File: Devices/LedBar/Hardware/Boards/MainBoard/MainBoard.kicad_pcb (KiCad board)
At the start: 2 copper layers, 99 x 24 mm, 115 parts, among them J201 12VDC/5A, J301 RS485, J401 AVR-ISP-6, J501 Left, J502 Center, J503 Right, J601 0-10V(1), Q501 Si2302DS, Q502 Si2302DS, Q503 Si2302DS, Q504 Si2302DS, Q505 Si2302DS, Q506 Si2302DS, Q507 Si2302DS, Q508 Si2302DS, Q509 Si2302DS, Q510 Si2302DS, Q511 Si2302DS, Q512 Si2302DS, Q513 Si2302DS, Q514 Si2302DS, Q515 Si2302DS, Q516 Si2302DS, SW401 reset, U201 INA219AxD, U202 AMS1117-5.0, U301 ISO3082DW, U302 B0505S-1W-SIP4, U401 ATmega48PV-10AU-arduino, U501 PCA9685PW, U701 LM393, Y401 14.7456Mhz

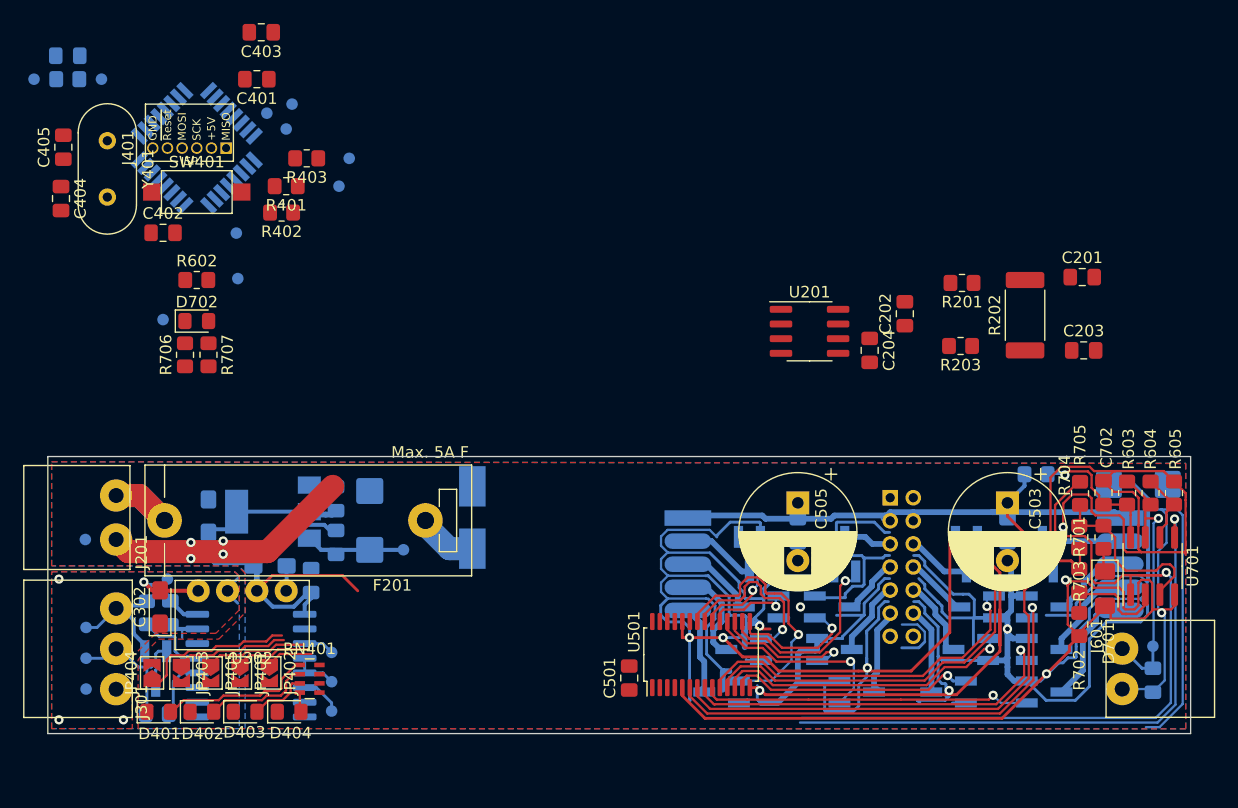
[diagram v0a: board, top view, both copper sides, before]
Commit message: Routing
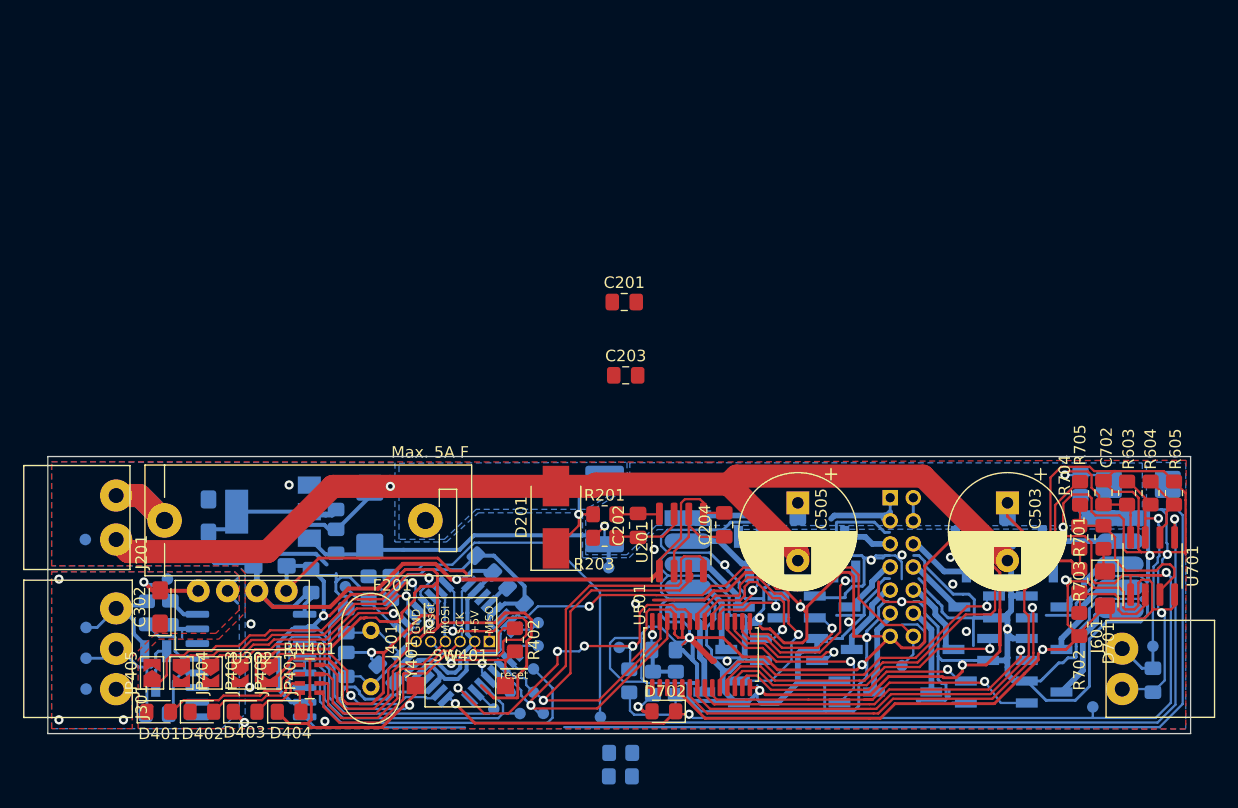
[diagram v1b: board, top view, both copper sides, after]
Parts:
- C401, C402, C403, C404, C405, C501, R202, R401, R403, R602, R706, R707: moved to B.Cu
- D201: moved to F.Cu
- moved TP701 87.3 mm to (190.5, 121.7), turned to 0 degrees
- moved TP603 73.9 mm to (147.9, 122.6), turned to 0 degrees
- moved TP405 71.8 mm to (174.0, 118.1), turned to 180 degrees
- moved R403 60.0 mm to (149.6, 127.7), turned to 0 degrees
- moved R401 57.0 mm to (149.6, 125.7), turned to 0 degrees
- moved C601 53.9 mm to (129.7, 111.4), turned to 270 degrees
- moved D702 52.7 mm to (153.4, 122.1), turned to 180 degrees
- moved TP402 51.8 mm to (142.5, 116.4), turned to 180 degrees
- moved R601 51.2 mm to (127.8, 111.4), turned to 270 degrees
- moved R706 51.2 mm to (154.4, 119.6), turned to 270 degrees
- moved R602 51.1 mm to (150.4, 119.4), turned to 90 degrees
- moved C401 50.1 mm to (140.6, 112.1), turned to 135 degrees
- moved C403 50.0 mm to (137.8, 109.3), turned to 315 degrees
- moved TP403 49.0 mm to (142.9, 122.2), turned to 180 degrees
- moved TP406 48.9 mm to (142.1, 120.4), turned to 180 degrees
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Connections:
- J401 pad 1: /Microcontroller/led3_miso -> /Microcontroller/led4_miso
- J401 pad 3: /Microcontroller/led4_sck -> /Microcontroller/led3_sck
- R402 pad 2: Net-(R402-Pad2) -> /Microcontroller/~reset~
- RN401 pad 5: /Microcontroller/led4_sck -> /Microcontroller/led4_miso
- RN401 pad 6: /Microcontroller/led3_miso -> /Microcontroller/led3_sck
- SW401 pad 2: Net-(R402-Pad2) -> /Microcontroller/~reset~
- U401 pad 16: /Microcontroller/led3_miso -> /Microcontroller/led4_miso
- U401 pad 17: /Microcontroller/led4_sck -> /Microcontroller/led3_sck
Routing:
- net GND: track 546.7 -> 1033.4 mm, vias 17 -> 35
- net +5V: track 38.1 -> 121.5 mm, vias 0 -> 2
- net /0-10V/a1: track 50.9 -> 102.6 mm
- net /Microcontroller/scl: track 0.00 -> 47.4 mm, vias 0 -> 1
- net /Microcontroller/~button~: track 0.00 -> 45.0 mm, vias 0 -> 1
- net /Brown-out/~Brown_out~: track 66.6 -> 109.3 mm, vias 1 -> 3
- net /Microcontroller/sda: track 0.00 -> 40.2 mm, vias 0 -> 1
- net /Microcontroller/led4_miso: track 0.00 -> 38.3 mm, vias 0 -> 1
- net /Pca/~oe~: track 0.00 -> 33.3 mm, vias 0 -> 4
- net /Microcontroller/tx_en: track 3.92 -> 33.5 mm
- net /Microcontroller/txd: track 3.59 -> 31.4 mm
- net /Microcontroller/rxd: track 2.65 -> 28.0 mm
- net /Microcontroller/led3_sck: track 0.00 -> 23.9 mm
- net /Microcontroller/addr5: track 8.78 -> 31.8 mm, vias 0 -> 1
- net /Microcontroller/led2_mosi: track 0.00 -> 22.2 mm
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- added copper zone on B.Cu, net +12V
- added copper zone on B.Cu, net Net-(C201-Pad1)
